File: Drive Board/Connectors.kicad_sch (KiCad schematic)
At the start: 0 parts

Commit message: Rev A of PCB
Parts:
- added J1: 1984620, Footprints:PHOENIX_1984620, symbol 1984620:1984620
- added J10, J9: B5B-XH-A, Footprints:JST_B5B-XH-A, symbol B5B-XH-A:B5B-XH-A
- added J11: Conn_01x04, Connector_PinHeader_2.54mm:PinHeader_1x04_P2.54mm_Vertical, symbol Connector_Generic:Conn_01x04
- added J2, J3, J4: 1984617, Footprints:PHOENIX_1984617, symbol 1984617:1984617
- added J5, J7, J8: B2B-XH-A, Footprints:JST_B2B-XH-A, symbol B2B-XH-A:B2B-XH-A
- added J6: B3B-XH-A, Footprints:JST_B3B-XH-A, symbol B3B-XH-A:B3B-XH-A
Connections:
- new net +24V: J4.1
- new net +3.3V: J11.1 (Pin_1)
- new net +5V: J10.1, J9.1
- new net BLDC A: J1.1
- new net BLDC B: J1.2
- new net BLDC C: J1.3
- new net BOOT: J6.1
- new net Brake_OUT1: J2.2
- new net Brake_OUT2: J2.1
- new net CANH: J6.2
- new net CANL: J6.3
- new net EncoderA_DO: J9.2
- new net EncoderA_PROG: J9.3
- new net EncoderB_DO: J10.2
- new net EncoderB_PROG: J10.3
- new net Encoder_CLK: J10.4, J9.4
- new net GND: J10.5, J11.4 (Pin_4), J4.2, J5.2, J7.2, J8.2, J9.5
- new net SWCLK: J11.2 (Pin_2)
- new net SWDIO: J11.3 (Pin_3)
- new net Steer_OUT1: J3.2
- new net Steer_OUT2: J3.1
- new net Temp BLDC Motor  : J5.1
- new net Temp Motor Brake: J7.1
- new net Temp Motor Steering: J8.1

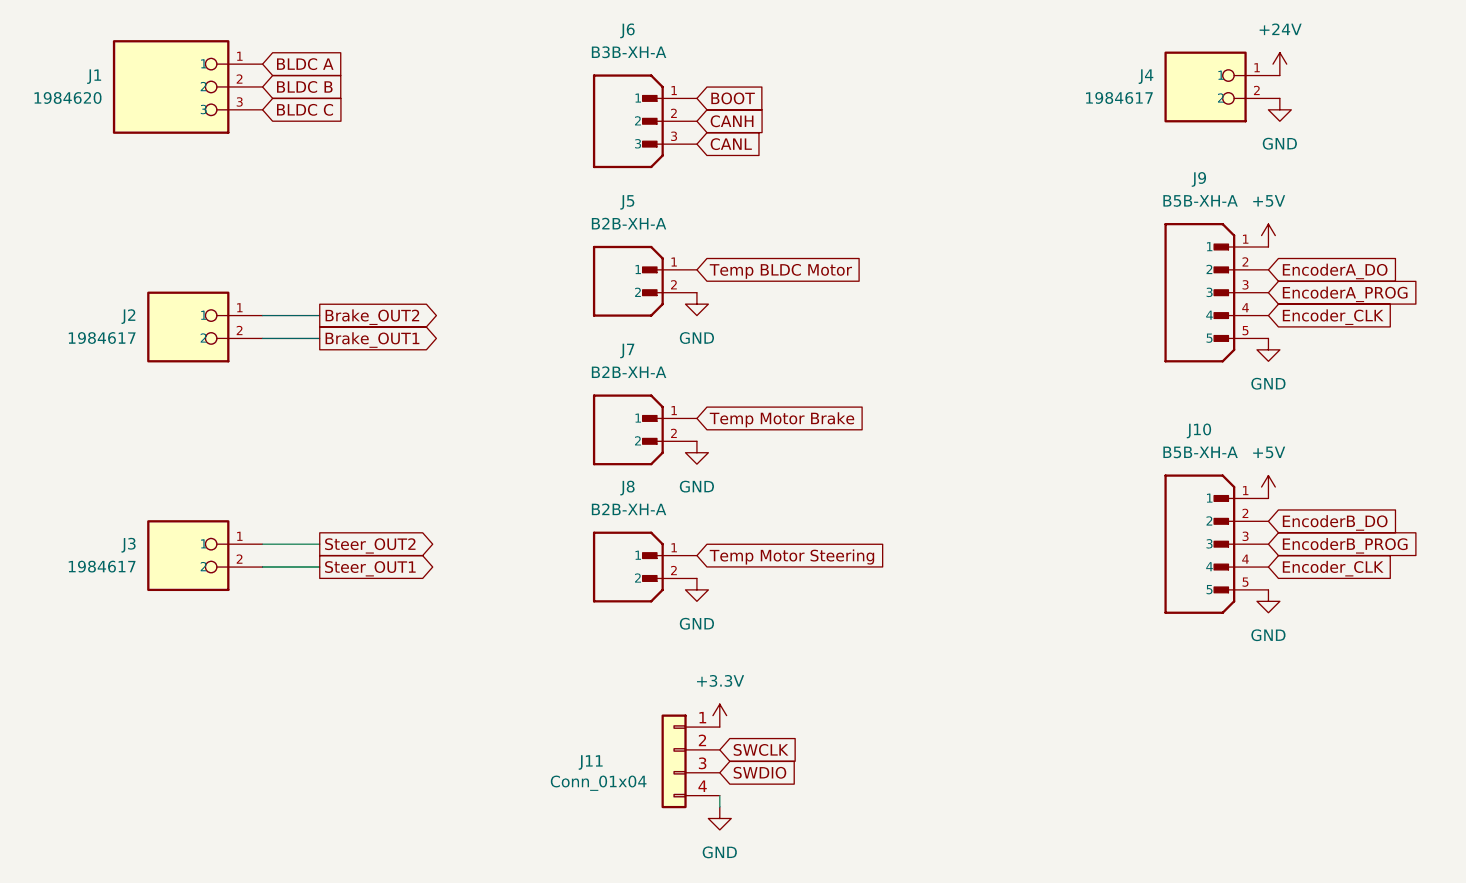
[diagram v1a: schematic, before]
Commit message: finished RV1 of board
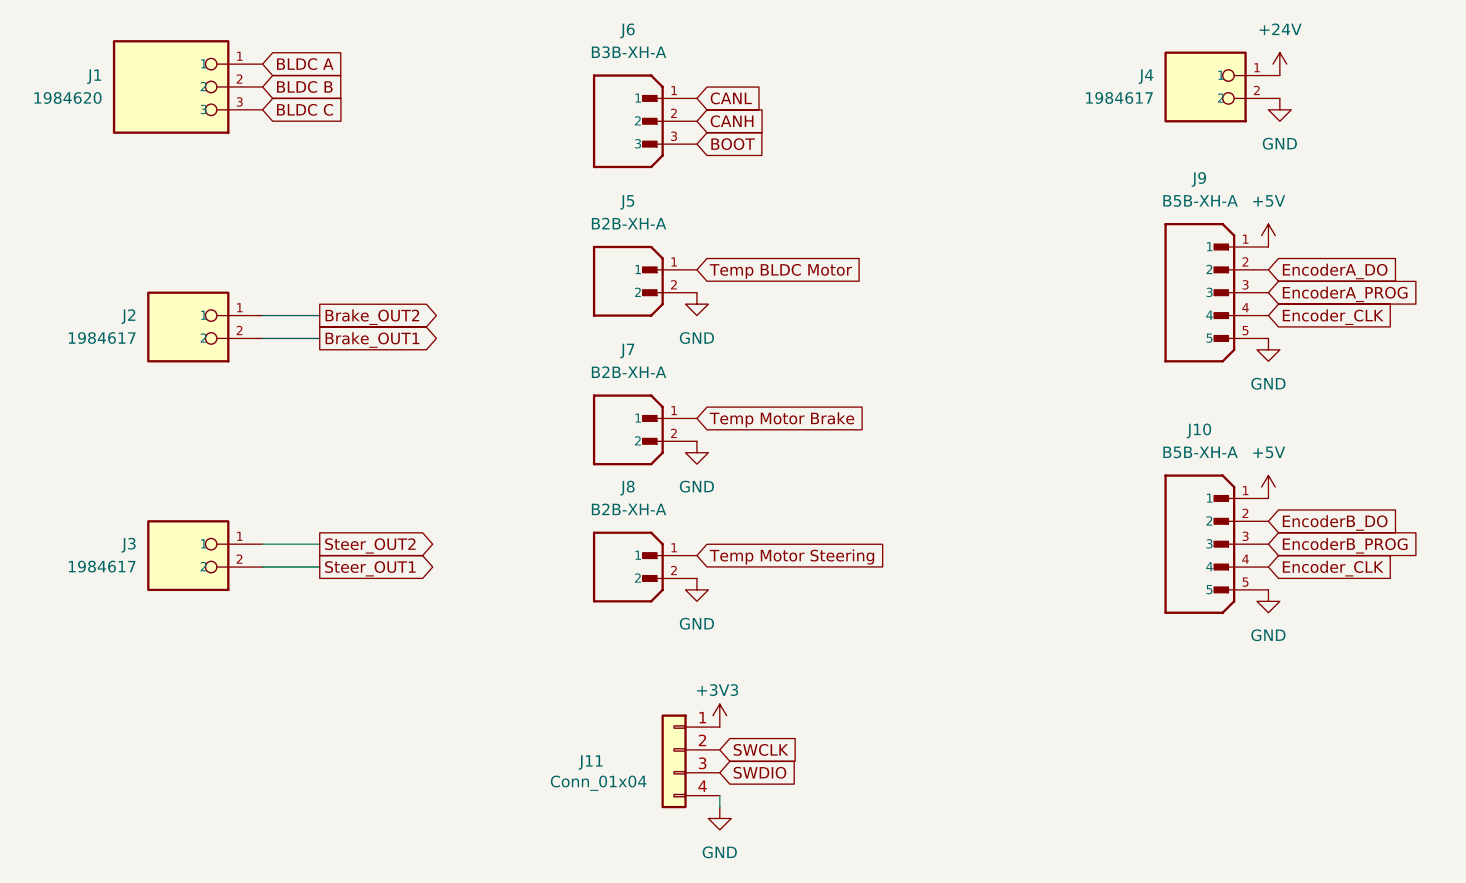
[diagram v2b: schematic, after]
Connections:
- net BOOT: now also J6.3; no longer J6.1
- net CANL: now also J6.1; no longer J6.3
- net +3.3V renamed +3V3
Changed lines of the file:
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@@
 	(global_label "BOOT"
 		(shape input)
-		(at 114.3 60.96 0)
+		(at 114.3 66.04 0)
 		(fields_autoplaced yes)
 		(effects
@@
 		)
 		(property "Intersheetrefs" "${INTERSHEET_REFS}"
-			(at 122.1838 60.96 0)
+			(at 122.1838 66.04 0)
 			(effects
 				(font
@@
 	(global_label "CANL"
 		(shape input)
-		(at 114.3 66.04 0)
+		(at 114.3 60.96 0)
 		(fields_autoplaced yes)
 		(effects
@@
 		)
 		(property "Intersheetrefs" "${INTERSHEET_REFS}"
-			(at 122.0024 66.04 0)
+			(at 122.0024 60.96 0)
 			(effects
 				(font
@@
 				(path "/3e208003-7c03-4e80-aaa5-209b125e5d65/4b37f0ac-bf6d-4a4a-8ba1-dd7985271430"
 					(reference "J1")
-					(unit 1)
-				)
-			)
-		)
-	)
-	(symbol
-		(lib_id "power:+3.3V")
-		(at 116.84 130.81 0)
-		(unit 1)
-		(exclude_from_sim no)
-		(in_bom yes)
-		(on_board yes)
-		(dnp no)
-		(fields_autoplaced yes)
-		(property "Reference" "#PWR081"
-			(at 116.84 134.62 0)
-			(effects
-				(font
-					(size 1.27 1.27)
-				)
-				(hide yes)
-			)
-		)
-		(property "Value" "+3.3V"
-			(at 116.84 125.73 0)
-			(effects
-				(font
-					(size 1.27 1.27)
-				)
-			)
-		)
-		(property "Footprint" ""
-			(at 116.84 130.81 0)
-			(effects
-				(font
-					(size 1.27 1.27)
-				)
-				(hide yes)
-			)
-		)
-		(property "Datasheet" ""
-			(at 116.84 130.81 0)
-			(effects
-				(font
-					(size 1.27 1.27)
-				)
-				(hide yes)
-			)
-		)
-		(property "Description" "Power symbol creates a global label with name \"+3.3V\""
-			(at 116.84 130.81 0)
-			(effects
-				(font
-					(size 1.27 1.27)
-				)
-				(hide yes)
-			)
-		)
-		(pin "1"
-		)
-		(instances
-			(project ""
-				(path "/3e208003-7c03-4e80-aaa5-209b125e5d65/4b37f0ac-bf6d-4a4a-8ba1-dd7985271430"
-					(reference "#PWR081")
 					(unit 1)
 				)
@@
 					(unit 1)
 				)
+			)
+		)
+	)
+	(symbol
+		(lib_id "power:+3V3")
+		(at 116.84 130.81 0)
+		(unit 1)
+		(exclude_from_sim no)
+		(in_bom yes)
+		(on_board yes)
+		(dnp no)
+		(property "Reference" "#PWR096"
+			(at 116.84 134.62 0)
+			(effects
+				(font
+					(size 1.27 1.27)
+				)
+				(hide yes)
+			)
+		)
+		(property "Value" "+3V3"
+			(at 116.586 126.746 0)
+			(effects
+				(font
+					(size 1.27 1.27)
+				)
+			)
+		)
+		(property "Footprint" ""
+			(at 116.84 130.81 0)
+			(effects
+				(font
+					(size 1.27 1.27)
+				)
+				(hide yes)
+			)
+		)
+		(property "Datasheet" ""
+			(at 116.84 130.81 0)
+			(effects
+				(font
+					(size 1.27 1.27)
+				)
+				(hide yes)
+			)
+		)
+		(property "Description" "Power symbol creates a global label with name \"+3V3\""
+			(at 116.84 130.81 0)
+			(effects
+				(font
+					(size 1.27 1.27)
+				)
+				(hide yes)
+			)
+		)
+		(pin "1"
+		)
+		(instances
+			(project "Drive Board"
+				(path "/3e208003-7c03-4e80-aaa5-209b125e5d65/4b37f0ac-bf6d-4a4a-8ba1-dd7985271430"
+					(reference "#PWR096")
+					(unit 1)
+				)
